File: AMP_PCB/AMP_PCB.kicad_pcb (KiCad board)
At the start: 2 copper layers, 25 x 25 mm, 23 parts, among them J1 Conn_Coaxial, J2 Conn_Coaxial, J3 Conn_Coaxial, J4 Conn_Coaxial, J5 Conn_01x02_Pin

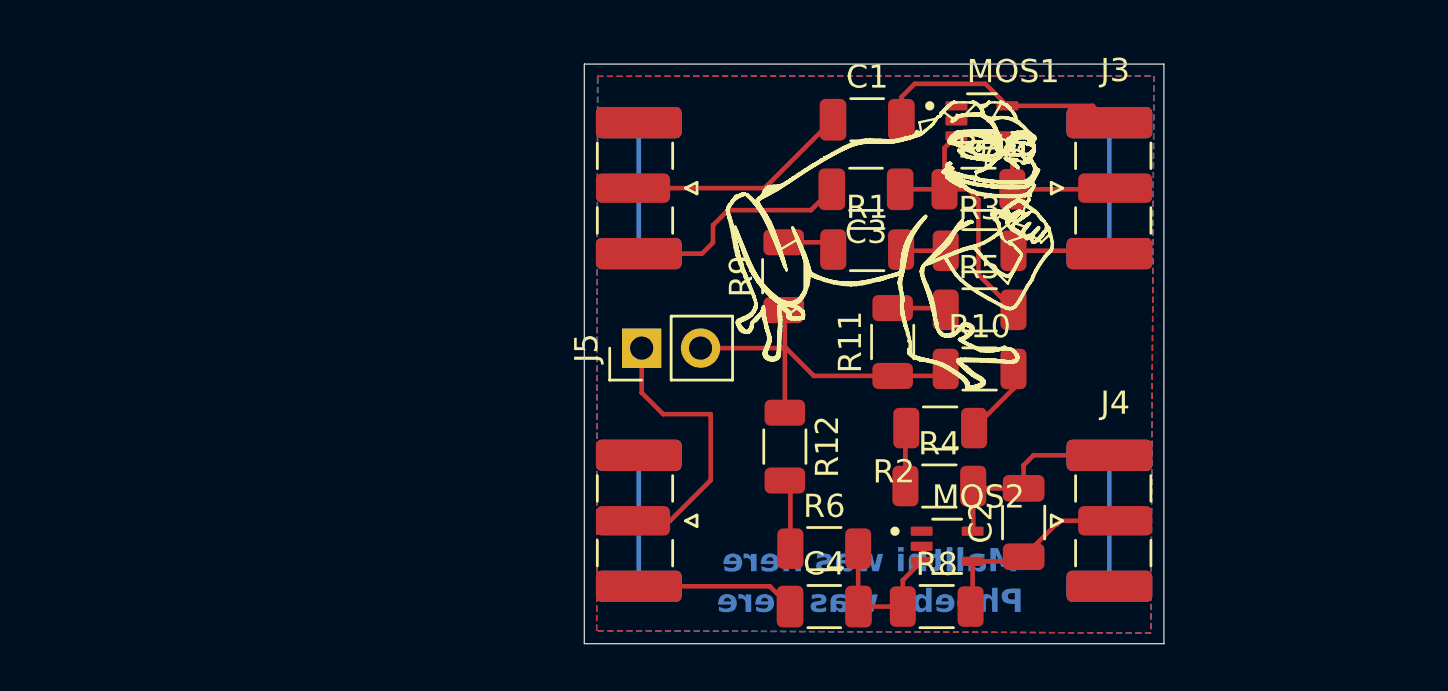
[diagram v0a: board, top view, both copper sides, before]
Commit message: etc
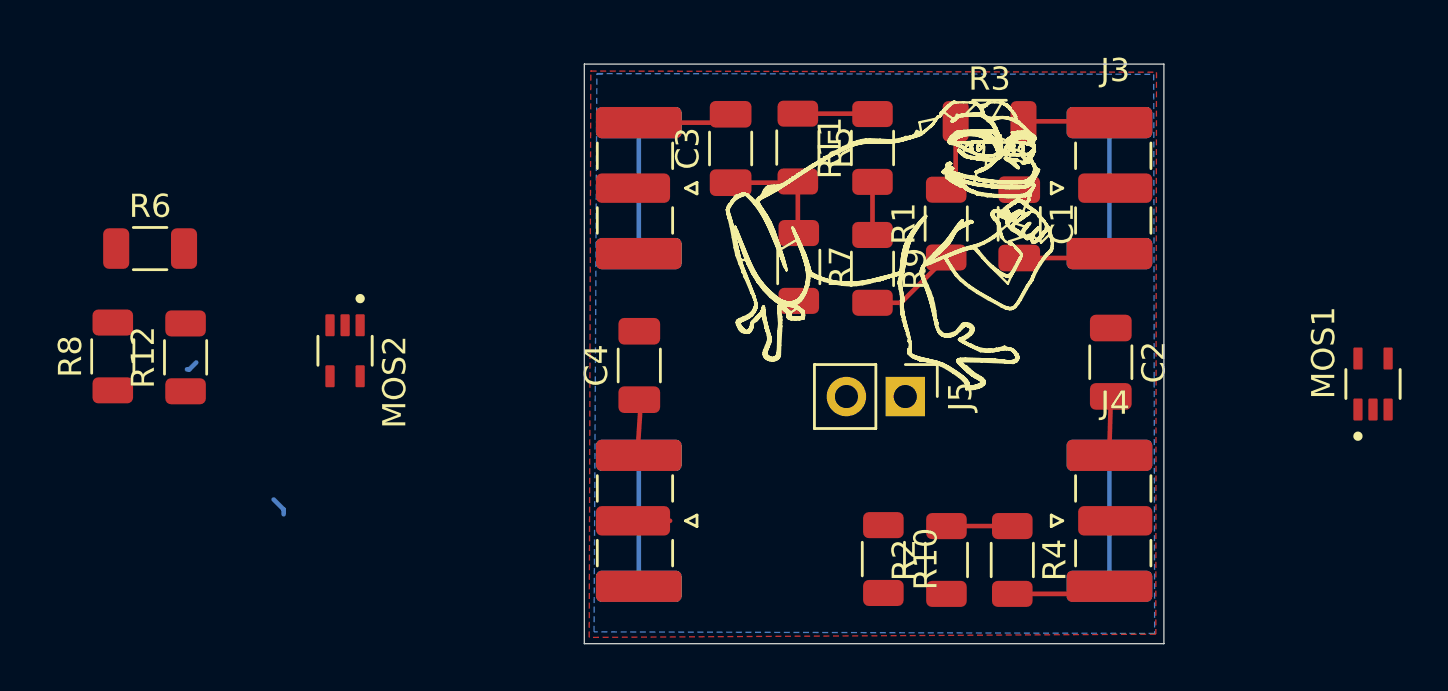
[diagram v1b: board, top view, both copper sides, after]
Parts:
- moved R8 37.1 mm to (79.7, 112.6), turned to 90 degrees
- moved R6 31.8 mm to (81.3, 108.0)
- moved MOS2 27.3 mm to (89.7, 112.4), turned to -90 degrees
- moved R12 26.1 mm to (82.8, 112.7), turned to 90 degrees
- moved MOS1 20.3 mm to (134.0, 113.8), turned to 90 degrees
- moved C4 13.1 mm to (102.4, 113.0), turned to 90 degrees
- moved J5 11.6 mm to (113.8, 114.3), turned to -90 degrees
- moved R5 10.5 mm to (109.2, 103.6), turned to -90 degrees
- moved R10 9.19 mm to (112.9, 121.3), turned to -90 degrees
- moved R7 8.44 mm to (109.2, 108.8), turned to -90 degrees
- moved R11 8.42 mm to (112.4, 103.6)
- moved C1 7.95 mm to (118.8, 106.9), turned to -90 degrees
- moved C2 7.87 mm to (122.7, 112.9), turned to -90 degrees
- moved C3 6.10 mm to (106.3, 103.6), turned to 90 degrees
- moved R2 5.70 mm to (115.6, 121.4), turned to 90 degrees
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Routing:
- net GND: track 37.8 -> 1.67 mm
- net Vdd: track 15.7 -> 2.29 mm
- net /Vout1: track 20.7 -> 13.5 mm
- net Vgate2: track 12.5 -> 5.65 mm
- net Net-(MOS2-G): track 6.70 -> 0.00 mm
- net Net-(MOS1-G): track 11.5 -> 5.16 mm
- net Vgate1: track 15.6 -> 9.76 mm
- net /Vout2: track 14.7 -> 9.98 mm
- net Net-(R10-Pad2): track 3.25 -> 0.00 mm
- net Net-(R12-Pad2): track 3.04 -> 0.00 mm
- net Net-(R1-Pad1): track 2.27 -> 3.99 mm
- net (no net): track 0.00 -> 1.34 mm
- net Net-(R1-Pad2): track 1.95 -> 3.12 mm
- net Net-(R11-Pad2): track 2.32 -> 3.23 mm
- added copper zone on B.Cu, net Vdd
- removed copper zone on B.Cu, net (none)
- removed copper zone on B.Cu, net GND
